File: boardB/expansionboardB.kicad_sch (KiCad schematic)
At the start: 46 parts, among them J1 USB_C_Receptacle, J3 HDMI_A, SW4 ESPPROG, U1 ESP32-S3-WROOM-1, U2 GPIO_U2, U4 GPIO_U4, U5 SII1136CTU, U7 MAX20022ATIA+T, t1V2 1V2_TEST, t3V3 3V3_TEST

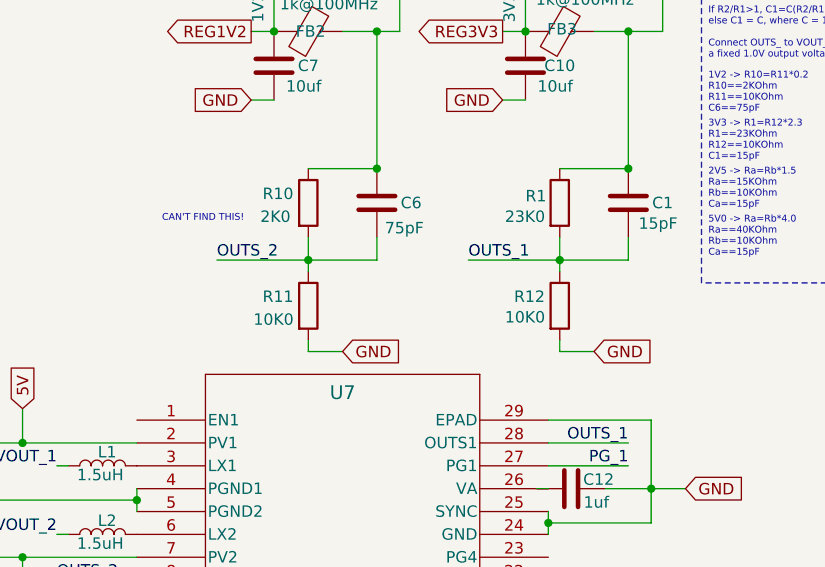
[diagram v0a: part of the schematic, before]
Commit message: Board updates
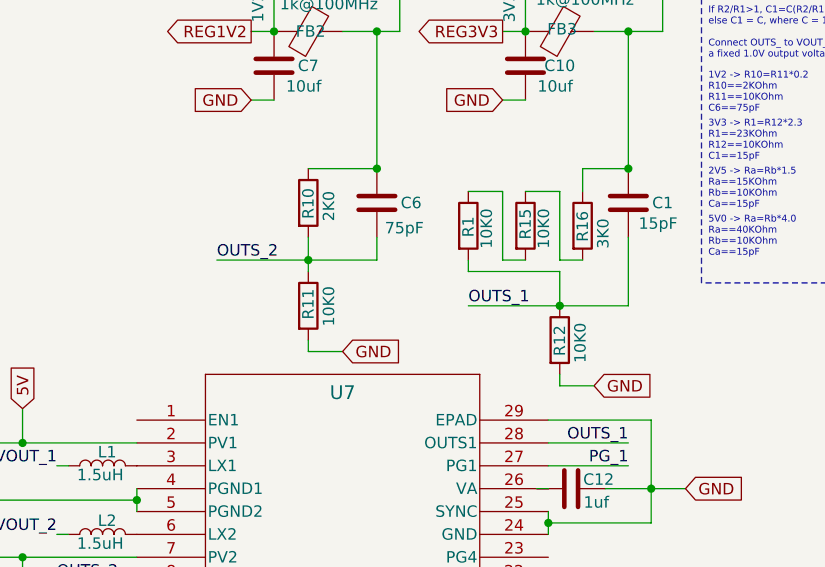
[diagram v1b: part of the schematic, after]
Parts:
- added R15: 10K0, Resistor_SMD:R_0603_1608Metric_Pad0.98x0.95mm_HandSolder, symbol Device:R
- added R16: 3K0, Resistor_SMD:R_0603_1608Metric_Pad0.98x0.95mm_HandSolder, symbol Device:R
- R1: value 23K0 -> 10K0
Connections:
- net VOUT_1: now also R16.1; no longer R1.1
- new net: R15.1, R16.2
- new net: R1.1, R15.2
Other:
- note removed: "CAN'T FIND THIS!"
- moved on the sheet: R1, R12
